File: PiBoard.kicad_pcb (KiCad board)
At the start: 4 copper layers, 74.2 x 101.4 mm, 129 parts, among them IC1 TCAN337DCNR, IC2 TPS2557QDRBTQ1, IC3 LM74502HDDFR, IC4 AP64501QSP-13, IC5 TPS2557QDRBTQ1, IC7 TPS2557QDRBTQ1, IC8 TPS2557QDRBTQ1, J1 CarLVPowerConnector, J10 USB_C_Receptacle, J11 RTC Battery Port, J14 4x nano-fit, J2 Display Breakout, J3 2222, J4 HDMI_D_1.4, J5 USB_C_Receptacle_USB2.0_16P, J6 CarCANConnector, J7 USB_C_Receptacle_USB2.0_16P, J8 CarCANConnector, Q2 NVMFWS1D7N04XMT1G, Q3 NVMFWS1D7N04XMT1G, SW1 SW_Push, SW2 SW_Push, U13 CDSOT23-T24CAN, U14 MCP2515-E/STVAO, Y4 8 MHz

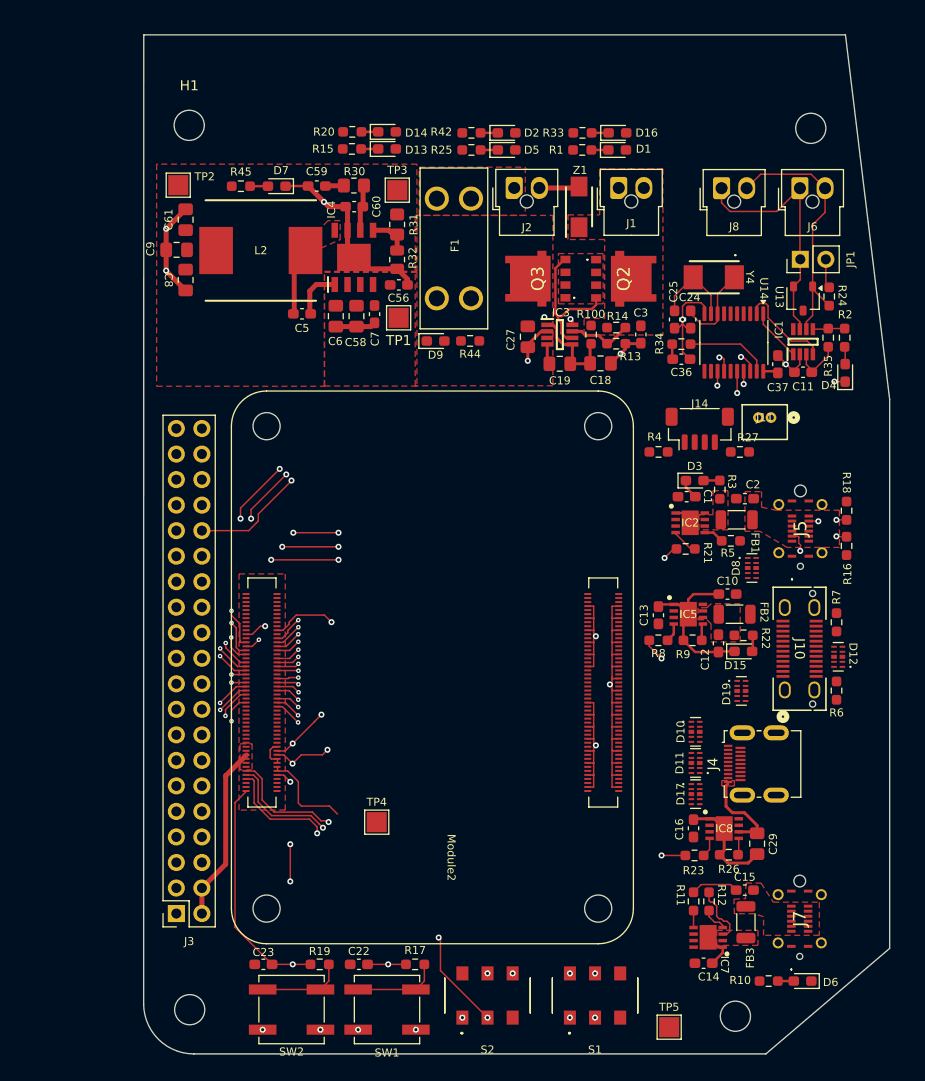
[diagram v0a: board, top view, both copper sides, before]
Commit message: frank2
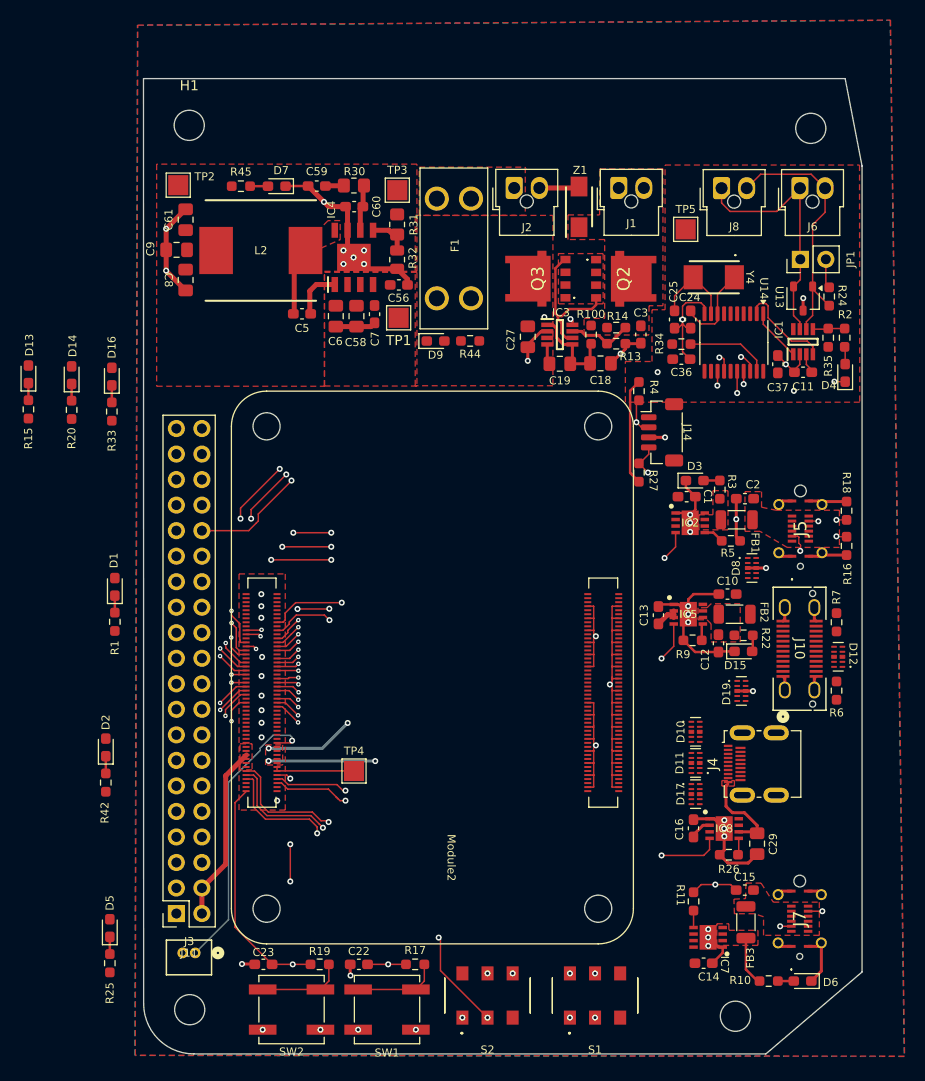
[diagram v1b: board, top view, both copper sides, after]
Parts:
- removed R12, R21, R23, R8: 100k, Resistor_SMD:R_0603_1608Metric_Pad0.98x0.95mm_HandSolder
- moved R25 88.6 mm to (58.4, 150.2), turned to -90 degrees
- moved D5 86.9 mm to (58.4, 146.7), turned to 90 degrees
- moved TP5 79.4 mm to (115.7, 77.2)
- moved J11 78.2 mm to (66.9, 149.2)
- moved R42 74.2 mm to (58.0, 132.2), turned to -90 degrees
- moved D2 73.0 mm to (58.0, 128.7), turned to 90 degrees
- moved D1 66.2 mm to (58.9, 112.7), turned to 90 degrees
- moved R1 66.1 mm to (58.9, 116.2), turned to -90 degrees
- moved D16 55.8 mm to (58.6, 91.8), turned to 90 degrees
- moved R33 54.4 mm to (58.6, 95.3), turned to -90 degrees
- moved D13 42.1 mm to (50.3, 91.6), turned to 90 degrees
- moved R15 41.3 mm to (50.3, 95.1), turned to -90 degrees
- moved D14 39.6 mm to (54.6, 91.7), turned to 90 degrees
- moved R20 39.3 mm to (54.6, 95.1), turned to -90 degrees
- moved R27 10.3 mm to (111.0, 101.3), turned to -90 degrees
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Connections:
- IC2 pad 4: Net-(IC2-EN) -> /CM5 GPIO/GLOBAL_EN
- IC5 pad 4: Net-(IC5-EN) -> /CM5 GPIO/GLOBAL_EN
- IC7 pad 4: Net-(IC7-EN) -> /High Speed/USB-C/VBUS_PWR
- IC8 pad 4: Net-(IC8-EN) -> /CM5 GPIO/GLOBAL_EN
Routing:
- net +3.3V: track 11.1 -> 167.4 mm, vias 0 -> 6
- net /CM5 GPIO/CC2: track 0.00 -> 77.8 mm, vias 0 -> 2
- net /CM5 GPIO/CC1: track 0.00 -> 66.3 mm, vias 0 -> 2
- net /CM5 GPIO/FAN_PWM: track 0.00 -> 55.2 mm, vias 0 -> 4
- net /CM5 GPIO/FAN_TACHO: track 0.00 -> 46.8 mm, vias 0 -> 2
- net GND: track 153.4 -> 195.2 mm, vias 19 -> 54
- net unconnected-(Module2A-SDA0-Pad82): track 29.1 -> 0.00 mm, vias 2 -> 0
- net /CM5 GPIO/RTC_Batt: track 0.00 -> 28.8 mm, vias 0 -> 1
- net unconnected-(Module2A-SCL0-Pad80): track 24.8 -> 0.00 mm, vias 2 -> 0
- net /CM5 GPIO/GLOBAL_EN: track 103.3 -> 110.1 mm
- net +5V: track 17.6 -> 22.4 mm
- net Net-(IC2-EN): track 2.65 -> 0.00 mm
- net Net-(IC7-EN): track 2.53 -> 0.00 mm
- net Net-(IC8-EN): track 1.94 -> 0.00 mm
- net Net-(IC5-EN): track 1.88 -> 0.00 mm
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- added copper zone on F.Cu, net +3.3V
- added copper zone on B.Cu, net GND
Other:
- board size 74.2 x 101.4 mm -> 71.5 x 97.1 mm
